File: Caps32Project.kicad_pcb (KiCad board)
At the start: 2 copper layers, 50 parts, among them J2 Sh 1.0, J3 USB_C_Receptacle_USB2.0_16P, Q2 AO3401A, SW1 Reset, SW2 Boot, U1 MPU-6050, U2 MAX17048G_T10, U3 ESP32-S2, U4 MCP73831-2-OT, U5 AP2112K-3.3, Y2 40MHz

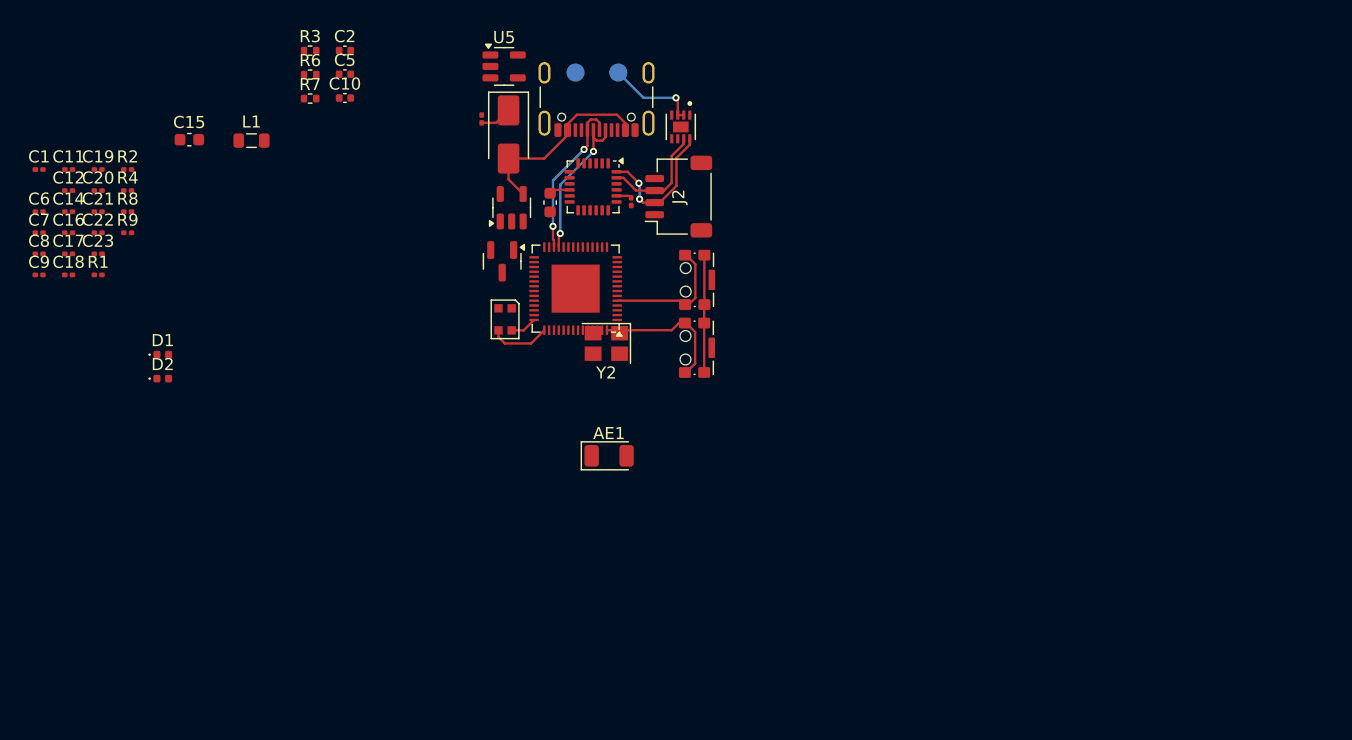
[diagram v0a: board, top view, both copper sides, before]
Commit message: Update Board
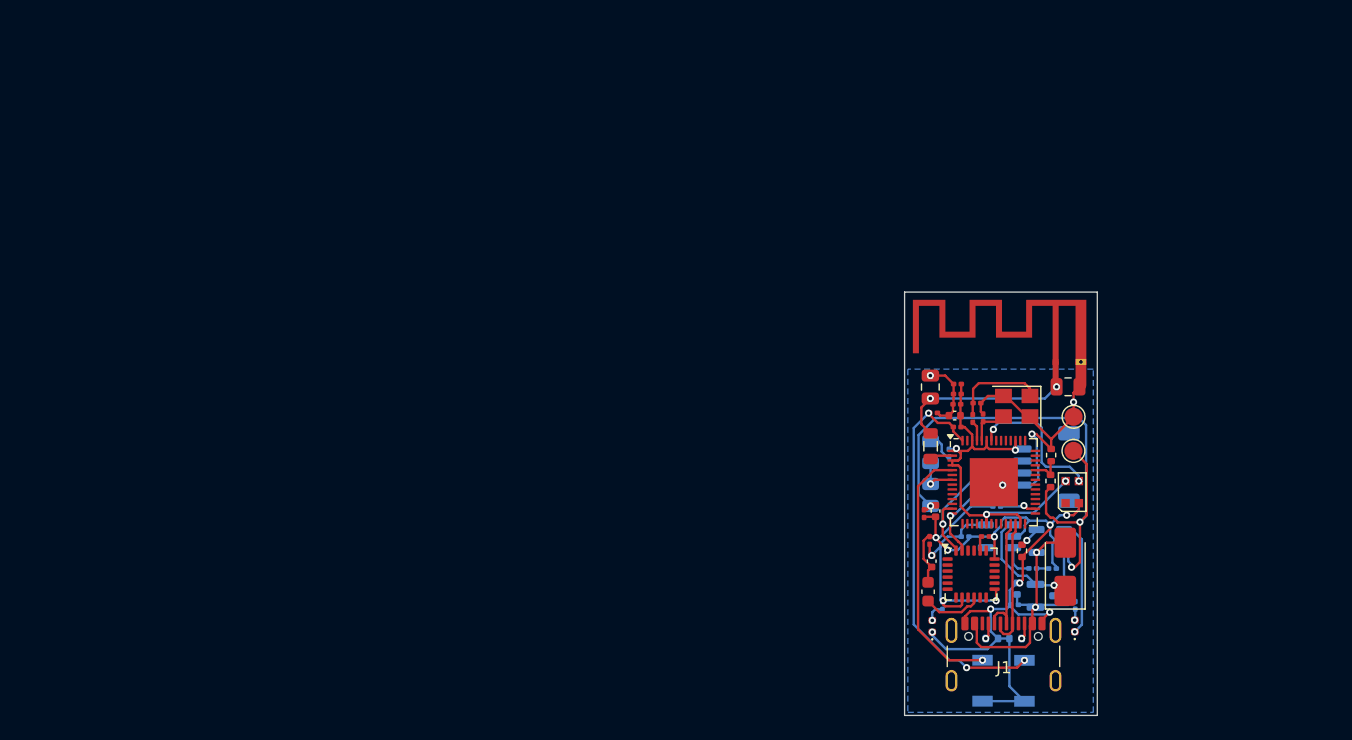
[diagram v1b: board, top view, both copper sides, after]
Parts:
- removed C22, C23: 1.0uF, Capacitor_SMD:C_0201_0603Metric
- removed D5: WS2812B-2020, LED_SMD:LED_WS2812B-2020_PLCC4_2.0x2.0mm
- removed J3: USB_C_Receptacle_USB2.0_16P, Connector_USB:USB_C_Receptacle_GCT_USB4105-xx-A_16P_TopMnt_Horizontal
- removed Q2: AO3401A, Package_TO_SOT_SMD:SOT-23
- removed U5: AP2112K-3.3, Package_TO_SOT_SMD:SOT-23-5
- removed Y2: 40MHz, Crystal:Crystal_SMD_3225-4Pin_3.2x2.5mm
- added C13: 0.1uF, Capacitor_SMD:C_0402_1005Metric, F.Cu at (141.5, 63.8)
- added D4: WS2812B-2020, LED_SMD:LED_WS2812B-2020_PLCC4_2.0x2.0mm, F.Cu at (151.2, 70.1)
- added J1: USB_C_Receptacle_USB2.0_16P, Connector_USB:USB_C_Receptacle_GCT_USB4105-xx-A_16P_TopMnt_Horizontal, F.Cu at (145.5, 84.7)
- added Q1: AO3401A, Package_TO_SOT_SMD:SOT-23, B.Cu at (149.1, 78.7)
- added R11: 160K, Resistor_SMD:R_0805_2012Metric, B.Cu at (139.5, 66.8)
- added R12: 3K3, Resistor_SMD:R_0402_1005Metric, F.Cu at (149.4, 69.2)
- added R13: 2K, Resistor_SMD:R_0402_1005Metric, F.Cu at (149.5, 67.0)
- added R5: 1K, Resistor_SMD:R_0201_0603Metric, B.Cu at (151.5, 79.5)
- added Y1: 40MHz, Crystal:Crystal_SMD_3225-4Pin_3.2x2.5mm, F.Cu at (146.6, 63.0)
- AE1: value Antenna_Chip -> Antenna; footprint RF_Antenna:Johanson_2450AT18x100 -> RF_Antenna:Texas_SWRA117D_2.4GHz_Left
- C1, C14, C19, J2, R1, R6, R7: moved to B.Cu
- C10: value 100pF -> 15pF; footprint Capacitor_SMD:C_0402_1005Metric -> Capacitor_SMD:C_0201_0603Metric
- C11: value 0.1uF -> 4.7uF; footprint Capacitor_SMD:C_0201_0603Metric -> Capacitor_SMD:C_0402_1005Metric
- C12: value 1uF -> 1.0uF
- C15: value 22uF -> 0.1uF; footprint Capacitor_SMD:C_0603_1608Metric -> Capacitor_SMD:C_0402_1005Metric
- C16: value 0.1uF -> 1uF
- C18: value 1uF -> 0.1uF; moved to B.Cu
- C2: value 4.7uF -> 0.1uF; footprint Capacitor_SMD:C_0402_1005Metric -> Capacitor_SMD:C_0805_2012Metric
- C20: value 0.1uF -> 1uF; moved to B.Cu
- C21: value 1.0uF -> 1uF
- C3: value 2.2nF -> 1uF; footprint Capacitor_SMD:C_0603_1608Metric -> Capacitor_SMD:C_0805_2012Metric
- C4: value 0.1uF -> 1.0uF
- C5: value 4.7uF -> 1.0uF; footprint Capacitor_SMD:C_0402_1005Metric -> Capacitor_SMD:C_0201_0603Metric
- C6: value 1uF -> 2.2nF; footprint Capacitor_SMD:C_0201_0603Metric -> Capacitor_SMD:C_0603_1608Metric
- C7: value 15pF -> 0.1uF
- C8: value 15pF -> 4.7uF; footprint Capacitor_SMD:C_0201_0603Metric -> Capacitor_SMD:C_0402_1005Metric; moved to B.Cu
- C9: value 1uF -> 15pF
- D2: value LED -> SS34; footprint LED_SMD:LED_0402_1005Metric -> Diode_SMD:D_SMA
- D3: value SS34 -> LED; footprint Diode_SMD:D_SMA -> LED_SMD:LED_0402_1005Metric
- L1: value 1.8nH -> ~
- R10: value 100K -> 442K; footprint Resistor_SMD:R_0201_0603Metric -> Resistor_SMD:R_0805_2012Metric; moved to B.Cu
- R2: value 1K -> 10K; moved to B.Cu
- R3: value 2K -> 100K; footprint Resistor_SMD:R_0402_1005Metric -> Resistor_SMD:R_0201_0603Metric; moved to B.Cu
- R4: value 10K -> 0
- R8: value 10K -> 2K; footprint Resistor_SMD:R_0201_0603Metric -> Resistor_SMD:R_0402_1005Metric
- R9: value 10K -> 100K
- SW1, SW2: footprint Button_Switch_SMD:SW_SPST_CK_KMS2xxGP -> Button_Switch_SMD:SW_SPST_B3U-1000P; moved to B.Cu
- TP1, TP2: moved to F.Cu
- U2: value MAX17048G_T10 -> AP2112K-3.3; footprint Custom:SON50P200X200X80-9N -> Package_TO_SOT_SMD:SOT-23-5; moved to B.Cu
- U3: value ESP32-S2 -> MCP73831-2-OT; footprint Package_DFN_QFN:QFN-56-1EP_7x7mm_P0.4mm_EP4x4mm -> Package_TO_SOT_SMD:SOT-23-5; moved to B.Cu
- U4: value MCP73831-2-OT -> ESP32-S2; footprint Package_TO_SOT_SMD:SOT-23-5 -> Package_DFN_QFN:QFN-56-1EP_7x7mm_P0.4mm_EP4x4mm
- moved C1 90.4 mm to (149.6, 76.5)
- moved C8 85.8 mm to (146.7, 78.1), turned to 90 degrees
- moved C7 82.5 mm to (144.0, 73.8)
- moved R2 82.0 mm to (146.5, 79.5), turned to 180 degrees
- moved C6 80.3 mm to (139.3, 78.4), turned to -90 degrees
- moved C19 79.4 mm to (145.0, 70.5), turned to 180 degrees
- moved R8 79.4 mm to (147.1, 75.0), turned to -90 degrees
- moved C20 79.1 mm to (145.0, 71.3), turned to 180 degrees
- moved C9 78.6 mm to (143.3, 62.7), turned to 180 degrees
- moved C18 77.5 mm to (142.3, 73.8)
- moved C11 77.4 mm to (139.9, 71.7), turned to -90 degrees
- moved D2 76.5 mm to (150.7, 76.3), turned to 90 degrees
- moved C12 75.9 mm to (138.9, 71.9), turned to -90 degrees
- moved C16 75.9 mm to (139.4, 74.1), turned to 90 degrees
- moved C14 75.8 mm to (141.0, 66.9), turned to -90 degrees
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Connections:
- C1 pad 1: +BATT -> Net-(D2-K)
- C10 pad 1: VDD3P3_CPU -> GND
- C10 pad 2: GND -> XTAL_N
- C11 pad 1: VDD3P3_CPU -> +BATT
- C12 pad 1: VDD3P3_CPU -> +BATT
- C14 pad 1: VDD3P3_CPU -> +3V3
- C15 pad 1: VDD3P3_CPU -> +3V3
- C16 pad 1: VDD3P3_CPU -> +3V3
- C17 pad 1: VDD_SPI -> +3V3
- C18 pad 1: VDD_SPI -> +3V3
- C19 pad 1: VDD3P3_CPU -> VDD_SPI
- C2 pad 1: VBUS -> GND
- C2 pad 2: GND -> Net-(AE1-FEED)
- C20 pad 1: VDD3P3_CPU -> VDD_SPI
- C21 pad 1: Net-(D3-K) -> RESET
- C3 pad 2: Net-(U1-REGOUT) -> Net-(AE1-FEED)
- C4 pad 1: Net-(U1-CPOUT) -> +3V3
- C5 pad 1: +BATT -> +3V3
- C6 pad 1: RESET -> GND
- C6 pad 2: GND -> Net-(U1-REGOUT)
- C7 pad 1: GND -> Net-(U1-CPOUT)
- C7 pad 2: Net-(C7-Pad2) -> GND
- C8 pad 1: GND -> VBUS
- C8 pad 2: Net-(U3-XTAL_P) -> GND
- C9 pad 1: VDD3P3_CPU -> GND
- C9 pad 2: GND -> Net-(C9-Pad2)
- D2 pad 2: Net-(D2-A) -> VBUS
- D3 pad 2: VBUS -> Net-(D3-A)
- J2 pad 1: VDD3P3_CPU -> +3V3
- L1 pad 1: VDD3P3 -> LNA
- L1 pad 2: VDD3P3_CPU -> Net-(AE1-FEED)
- R1 pad 1: VDD3P3_CPU -> +3V3
- R10 pad 1: Net-(D3-K) -> +BATT
- R10 pad 2: Net-(U5-EN) -> IO2
- R2 pad 2: Net-(D2-A) -> GND
- R3 pad 1: Net-(U4-PROG) -> Net-(D2-K)
- R3 pad 2: GND -> Net-(U2-EN)
- R4 pad 1: Net-(C7-Pad2) -> Net-(C9-Pad2)
- R4 pad 2: Net-(U3-XTAL_N) -> XTAL_P
- R8 pad 1: VDD3P3_CPU -> Net-(U3-PROG)
- R8 pad 2: RESET -> GND
- R9 pad 1: VBUS -> +3V3
- R9 pad 2: GND -> RESET
- U1 pad 13: VDD3P3_CPU -> +3V3
- U1 pad 8: VDD3P3_CPU -> +3V3
- U2 pad 1: GND -> Net-(D2-K)
- U2 pad 2: +BATT -> GND
- U2 pad 3: +BATT -> Net-(U2-EN)
- U2 pad 4: GND -> unconnected-(U2-NC-Pad4)
- U2 pad 5: unconnected-(U2-~{ALERT}-Pad5) -> +3V3
- U3 pad 1: VDD3P3_CPU -> Net-(D3-K)
- U3 pad 2: Net-(AE1-FEED) -> GND
- U3 pad 3: VDD3P3 -> +BATT
- U3 pad 4: VDD3P3 -> VBUS
- U3 pad 5: BOOT -> Net-(U3-PROG)
- U4 pad 1: Net-(D2-K) -> +3V3
- U4 pad 2: GND -> LNA
- U4 pad 3: +BATT -> +3V3
- U4 pad 4: VBUS -> +3V3
- U4 pad 5: Net-(U4-PROG) -> BOOT
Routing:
- net GND: track 9.74 -> 112.8 mm, vias 0 -> 13
- net +3V3: track 0.00 -> 56.4 mm, vias 0 -> 7
- net +BATT: track 7.65 -> 52.0 mm, vias 1 -> 3
- net RESET: track 11.6 -> 33.1 mm, vias 0 -> 3
- net Net-(AE1-FEED): track 0.00 -> 16.5 mm, vias 0 -> 2
- net RGB: track 0.00 -> 12.3 mm, vias 0 -> 2
- net Net-(D2-K): track 0.00 -> 12.2 mm, vias 0 -> 1
- net BOOT: track 10.8 -> 21.7 mm, vias 0 -> 1
- net Net-(C9-Pad2): track 0.00 -> 7.86 mm
- net Net-(D3-K): track 2.66 -> 9.74 mm, vias 0 -> 1
- net VBUS: track 16.1 -> 22.7 mm, vias 0 -> 2
- net NEO_D: track 5.04 -> 0.00 mm
- net VDD_SPI: track 0.00 -> 3.82 mm, vias 0 -> 1
- net IO2: track 0.00 -> 3.69 mm, vias 0 -> 1
- net XTAL_N: track 0.00 -> 3.49 mm
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- added copper zone on B.Cu, net GND
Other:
- board outline added: 16 x 35.1 mm

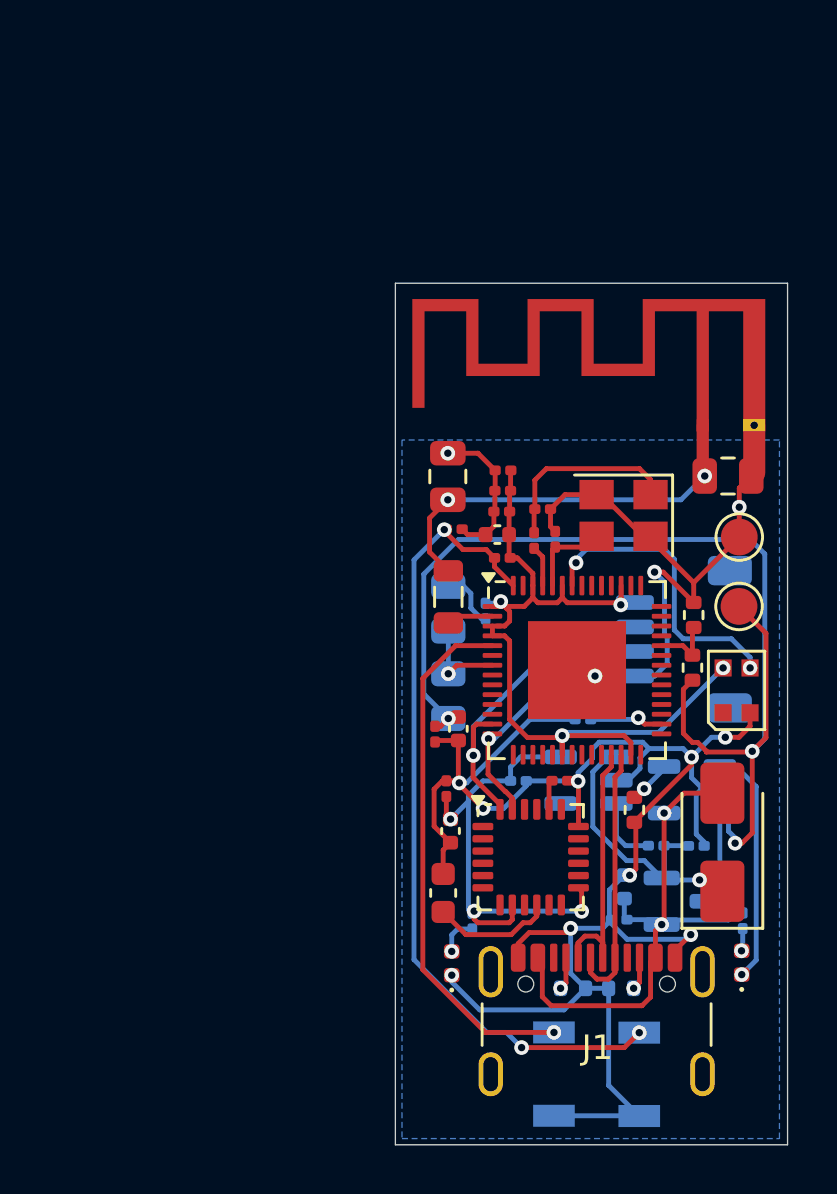
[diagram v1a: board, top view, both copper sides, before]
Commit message: Board Update
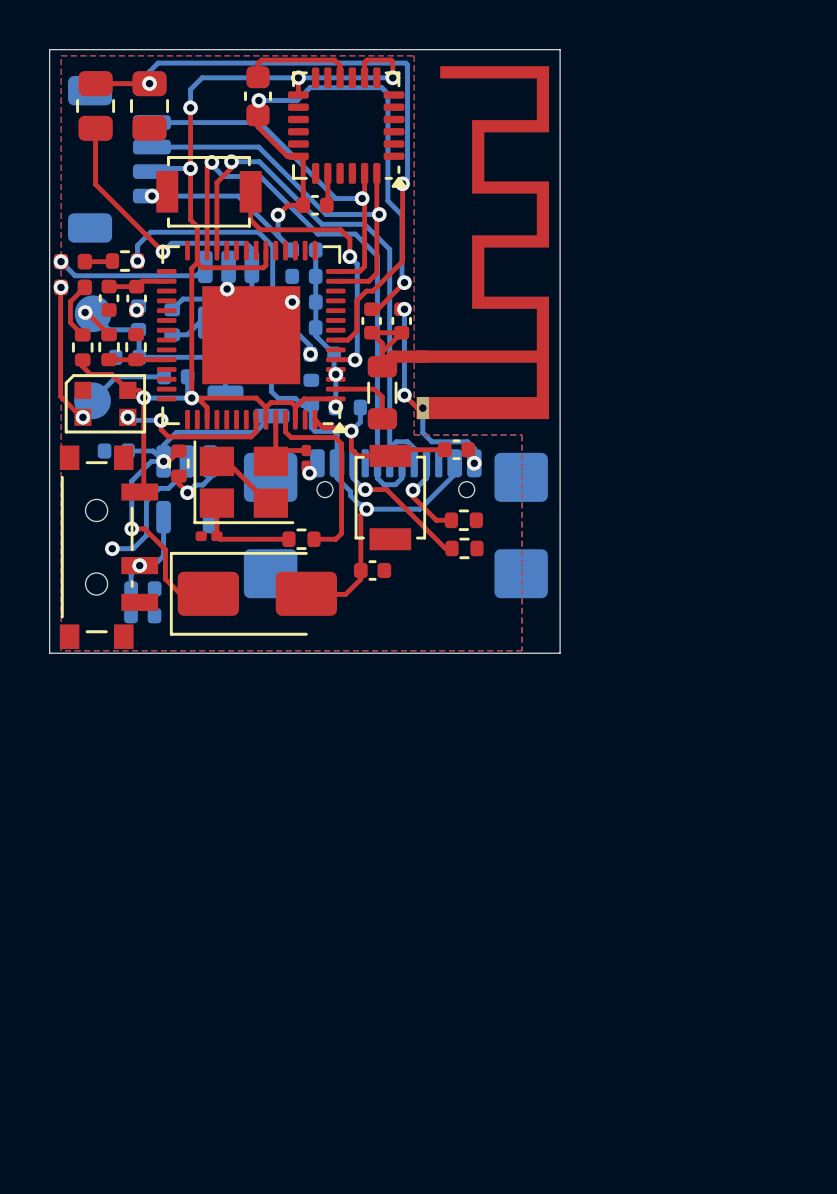
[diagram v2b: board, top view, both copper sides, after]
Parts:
- added SW3: SW_SPDT, Button_Switch_SMD:SW_SPDT_PCM12, F.Cu at (125.5, 64.3)
- C1, C14, C18, C21, C7: footprint Capacitor_SMD:C_0201_0603Metric -> Capacitor_SMD:C_0402_1005Metric
- C11, C13, C15, R8, TP1, TP2: moved to B.Cu
- C12, C16, C17, C4, C5: footprint Capacitor_SMD:C_0201_0603Metric -> Capacitor_SMD:C_0402_1005Metric; moved to B.Cu
- C19, C20: footprint Capacitor_SMD:C_0201_0603Metric -> Capacitor_SMD:C_0402_1005Metric; moved to F.Cu
- C2, C3: footprint Capacitor_SMD:C_0805_2012Metric -> Capacitor_SMD:C_0402_1005Metric
- C8, R10, R11, R6, R7, SW1, SW2: moved to F.Cu
- J1: footprint Connector_USB:USB_C_Receptacle_GCT_USB4105-xx-A_16P_TopMnt_Horizontal -> Connector_USB:USB_C_Receptacle_GCT_USB4110; moved to B.Cu
- J2: value Sh 1.0 -> SH1.0; footprint Connector_JST:JST_SH_SM04B-SRSS-TB_1x04-1MP_P1.00mm_Horizontal -> Connector_JST:JST_SH_BM04B-SRSS-TB_1x04-1MP_P1.00mm_Vertical
- R1, R3, R5: footprint Resistor_SMD:R_0201_0603Metric -> Resistor_SMD:R_0402_1005Metric; moved to F.Cu
- R2, R4: footprint Resistor_SMD:R_0201_0603Metric -> Resistor_SMD:R_0402_1005Metric
- R9: footprint Resistor_SMD:R_0201_0603Metric -> Resistor_SMD:R_0402_1005Metric; moved to B.Cu
- moved D3 39.5 mm to (124.2, 52.6), turned to 0 degrees
- moved SW2 38.6 mm to (129.7, 49.8), turned to 0 degrees
- moved R5 36.9 mm to (126.3, 52.6), turned to 180 degrees
- moved C6 33.4 mm to (131.7, 45.9), turned to 90 degrees
- moved D1 31.6 mm to (124.2, 53.7), turned to 0 degrees
- moved U1 30.8 mm to (135.3, 47.1), turned to 180 degrees
- moved J2 30.2 mm to (126.1, 48.5)
- moved TP1 28.9 mm to (125.0, 54.8), turned to 180 degrees
- moved C1 28.6 mm to (125.9, 60.4), turned to 180 degrees
- moved R1 28.3 mm to (124.6, 56.1), turned to 90 degrees
- moved D4 28.3 mm to (125.5, 58.4), turned to 0 degrees
- moved R10 28.0 mm to (125.1, 46.3)
- moved U3 27.7 mm to (130.5, 54.0), turned to -90 degrees
- moved R8 27.4 mm to (128.2, 55.1), turned to 90 degrees
- moved Q1 27.3 mm to (131.3, 58.0), turned to 180 degrees
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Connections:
- C4 pad 1: +3V3 -> Net-(SW3-B)
- C5 pad 1: +3V3 -> Net-(SW3-B)
- J2 pad 1: +3V3 -> SCL
- J2 pad 3: SCL -> +3V3
- J2 pad MP: (no net) -> GND
- U2 pad 5: +3V3 -> Net-(SW3-B)
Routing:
- net GND: track 112.8 -> 61.9 mm, vias 13 -> 15
- net +BATT: track 52.0 -> 26.0 mm, vias 3 -> 2
- net RESET: track 33.1 -> 7.56 mm, vias 3 -> 1
- net IO2: track 3.69 -> 26.3 mm, vias 1 -> 2
- net USB_P: track 10.8 -> 23.0 mm, vias 0 -> 1
- net USB_N: track 10.9 -> 23.0 mm, vias 0 -> 1
- net BOOT: track 21.7 -> 11.4 mm, vias 1 -> 2
- net Net-(AE1-FEED): track 16.5 -> 7.25 mm, vias 2 -> 0
- net VBUS: track 22.7 -> 31.2 mm
- net XTAL_P: track 1.66 -> 7.86 mm
- net RGB: track 12.3 -> 6.37 mm
- net Net-(SW3-B): track 0.00 -> 4.91 mm, vias 0 -> 1
- net Net-(J1-CC2): track 1.35 -> 5.84 mm
- net Net-(D2-K): track 12.2 -> 16.5 mm, vias 1 -> 2
- net SCL: track 11.0 -> 15.1 mm
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- added copper zone on F.Cu, net GND
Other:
- board size 16 x 35.1 mm -> 20.8 x 24.6 mm
